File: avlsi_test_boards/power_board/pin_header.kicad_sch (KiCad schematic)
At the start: 4 parts, among them J5 Conn_02x20_Odd_Even, J6 Conn_02x20_Odd_Even, J7 Conn_02x20_Odd_Even, J8 Conn_02x20_Odd_Even

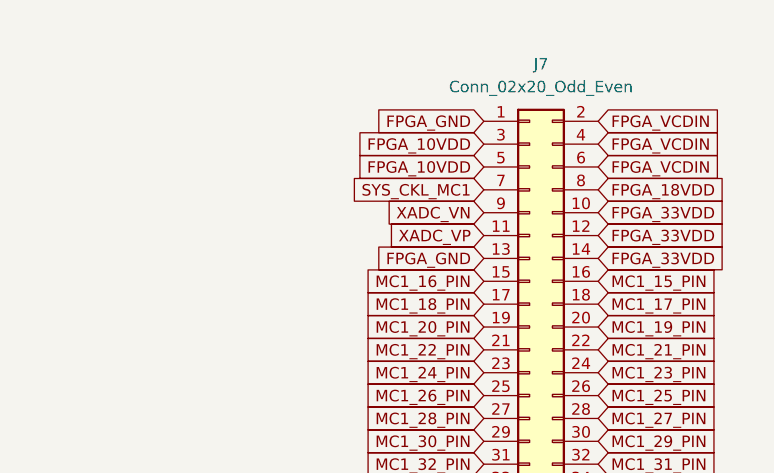
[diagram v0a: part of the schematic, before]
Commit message: Add fix typo
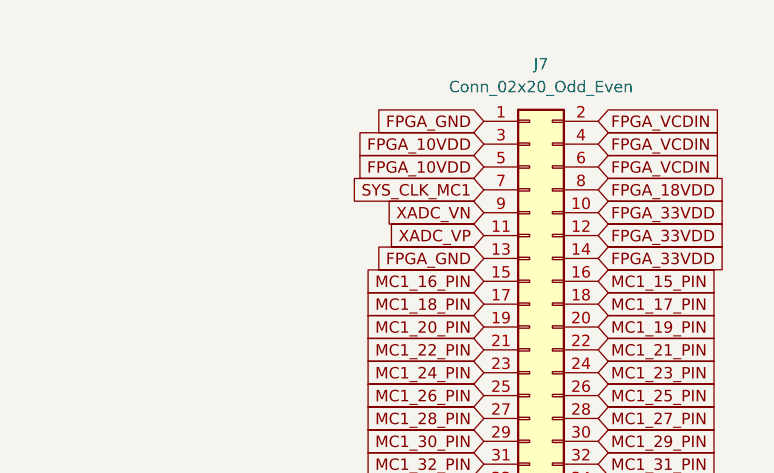
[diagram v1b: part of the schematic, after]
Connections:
- net SYS_CKL_MC1 renamed SYS_CLK_MC1
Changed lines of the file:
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@@
 		)
 	)
-	(global_label "SYS_CKL_MC1"
+	(global_label "SYS_CLK_MC1"
 		(shape input)
 		(at 222.25 40.64 180)
